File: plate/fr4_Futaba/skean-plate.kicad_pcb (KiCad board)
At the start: 2 copper layers, 153.2 x 95.3 mm, 16 parts

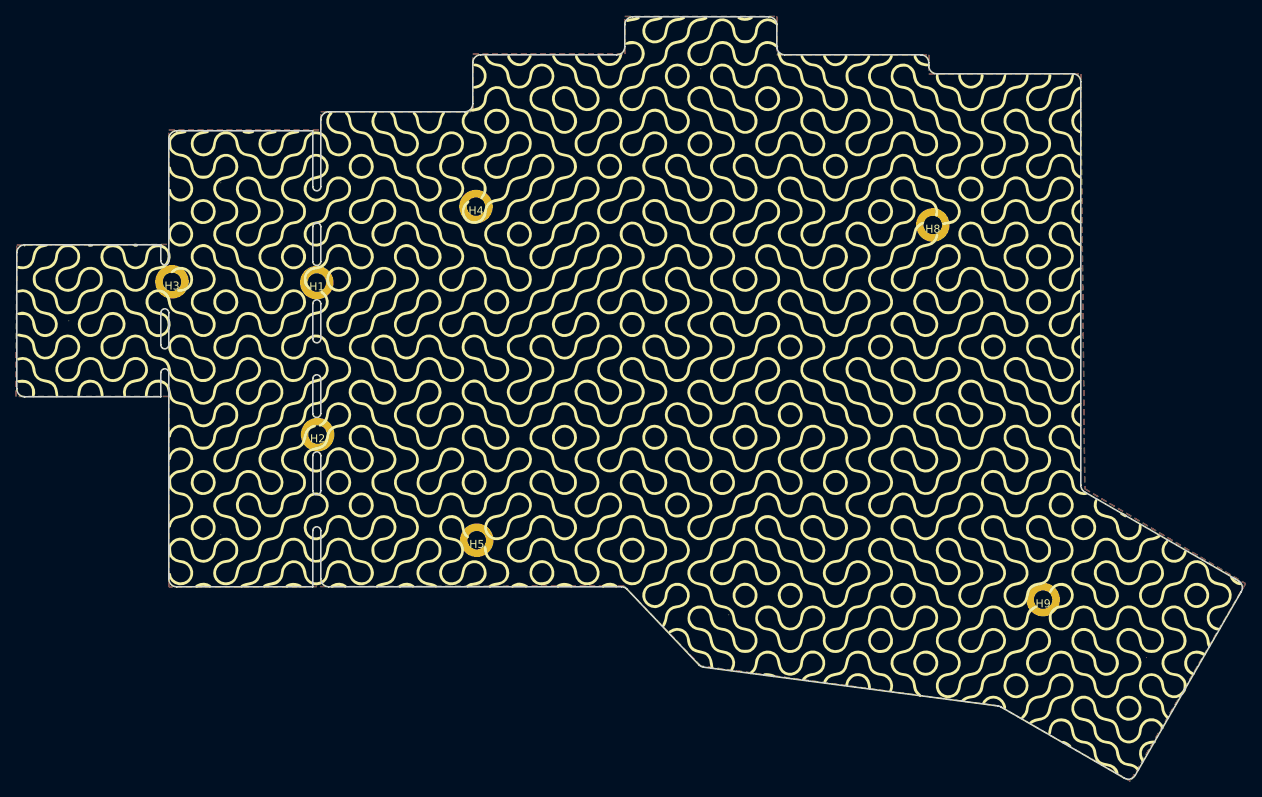
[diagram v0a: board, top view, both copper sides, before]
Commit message: V0.3 case files
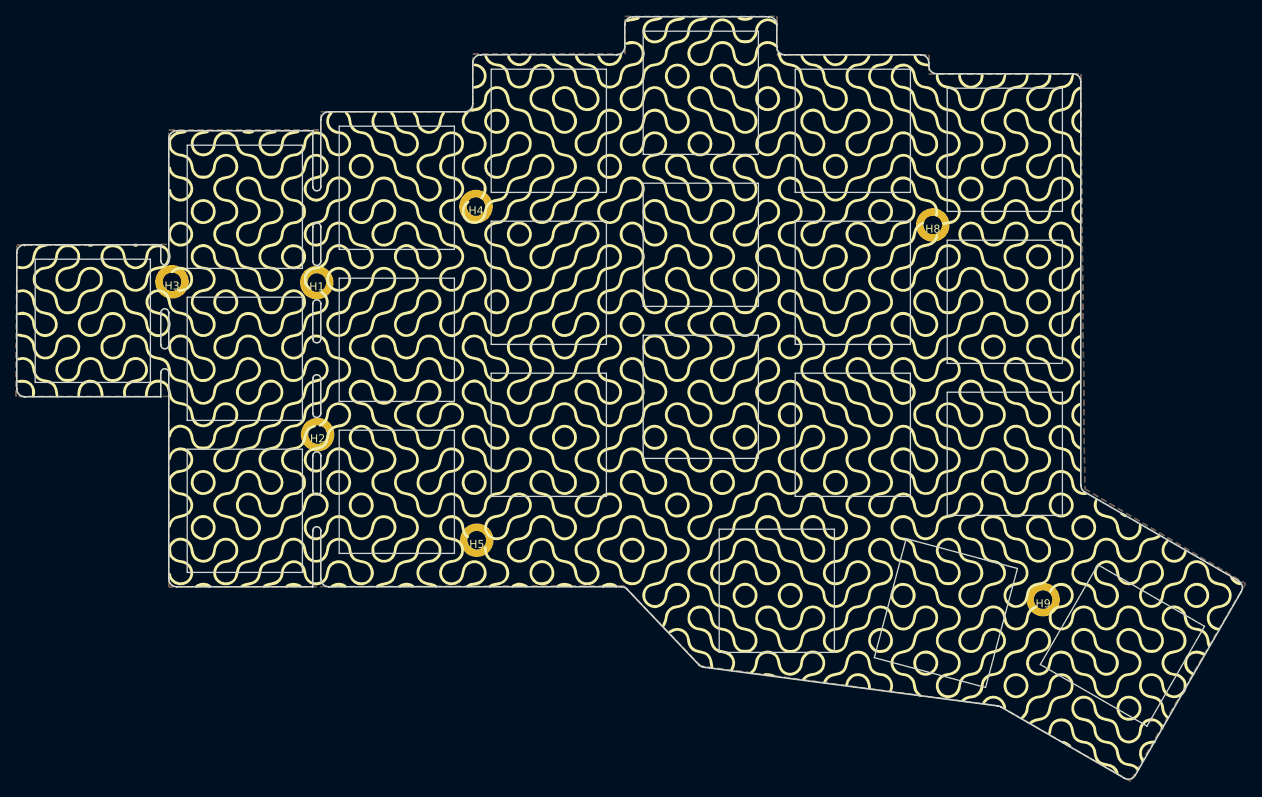
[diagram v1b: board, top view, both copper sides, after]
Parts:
- removed the REF** at (39.7, 35.1)
- removed the REF** at (140.7, 28.0)
- removed the REF** at (155.4, 94.4)
- removed the REF** at (39.7, 79.1)
- removed the REF** at (99.7, 20.8)
- removed the REF** at (20.7, 52.3)
- removed the REF** at (103.2, 89.1)
- added K1: KEYSW, kbd:SW_Hole_Futaba_MA, F.Cu at (130.4, 88.9)
- added K10: KEYSW, kbd:SW_Hole_Futaba_MA, F.Cu at (23.7, 52.3)
- added K11: KEYSW, kbd:SW_Hole_Futaba_MA, F.Cu at (99.7, 23.8)
- added K12: KEYSW, kbd:SW_Hole_Futaba_MA, F.Cu at (118.7, 66.6)
- added K13: KEYSW, kbd:SW_Hole_Futaba_MA, F.Cu at (61.7, 35.7)
- added K14: KEYSW, kbd:SW_Hole_Futaba_MA, F.Cu at (42.7, 57.1)
- added K15: KEYSW, kbd:SW_Hole_Futaba_MA, F.Cu at (99.7, 61.8)
- added K16: KEYSW, kbd:SW_Hole_Futaba_MA, F.Cu at (118.7, 28.6)
- added K17: KEYSW, kbd:SW_Hole_Futaba_MA, F.Cu at (61.7, 54.7)
- added K18: KEYSW, kbd:SW_Hole_Futaba_MA, F.Cu at (42.7, 76.1)
- added K19: KEYSW, kbd:SW_Hole_Futaba_MA, F.Cu at (99.7, 42.8)
- added K2: KEYSW, kbd:SW_Hole_Futaba_MA, F.Cu at (137.7, 69.0)
- added K20: KEYSW, kbd:SW_Hole_Futaba_MA, F.Cu at (80.7, 28.6)
- added K21: KEYSW, kbd:SW_Hole_Futaba_MA, F.Cu at (118.7, 47.6)
- added K22: KEYSW, kbd:SW_Hole_Futaba_MA, F.Cu at (152.4, 92.9)
- added K3: KEYSW, kbd:SW_Hole_Futaba_MA, F.Cu at (137.7, 50.0)
- added K4: KEYSW, kbd:SW_Hole_Futaba_MA, F.Cu at (137.7, 31.0)
- added K5: KEYSW, kbd:SW_Hole_Futaba_MA, F.Cu at (109.2, 86.1)
- added K6: KEYSW, kbd:SW_Hole_Futaba_MA, F.Cu at (80.7, 47.6)
- added K7: KEYSW, kbd:SW_Hole_Futaba_MA, F.Cu at (42.7, 38.1)
- added K8: KEYSW, kbd:SW_Hole_Futaba_MA, F.Cu at (61.7, 73.7)
- added K9: KEYSW, kbd:SW_Hole_Futaba_MA, F.Cu at (80.7, 66.6)
